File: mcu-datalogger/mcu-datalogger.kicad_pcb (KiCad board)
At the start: 2 copper layers, 29 parts, among them J1 Conn_01x04_Pin, J2 Conn_01x04_Pin, J3 Conn_01x09_Pin, J4 Conn_02x03_Odd_Even, U1 24LC1025, U2 24LC1025, U3 DS1337S_, U4 ATMEGA328P-AU, Y1 16MHz, Y2 32.768 KHz

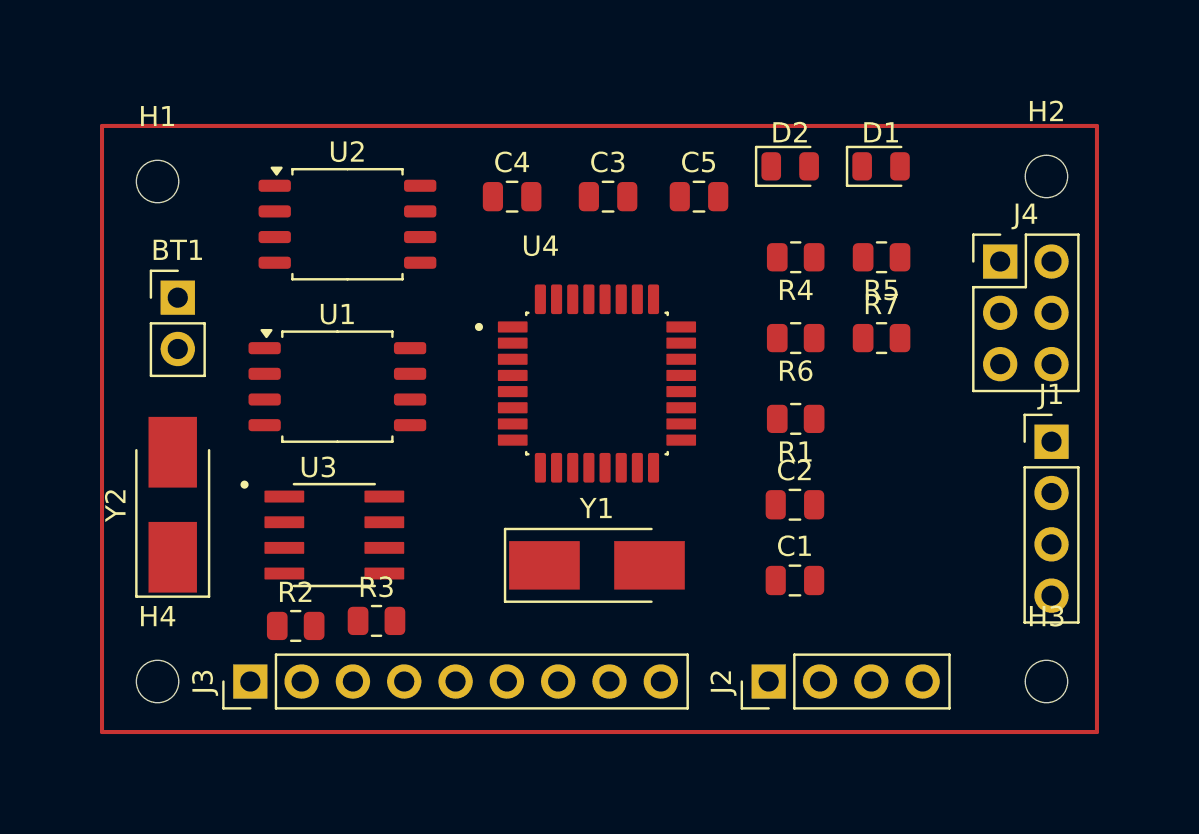
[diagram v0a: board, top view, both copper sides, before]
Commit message: routed pcb
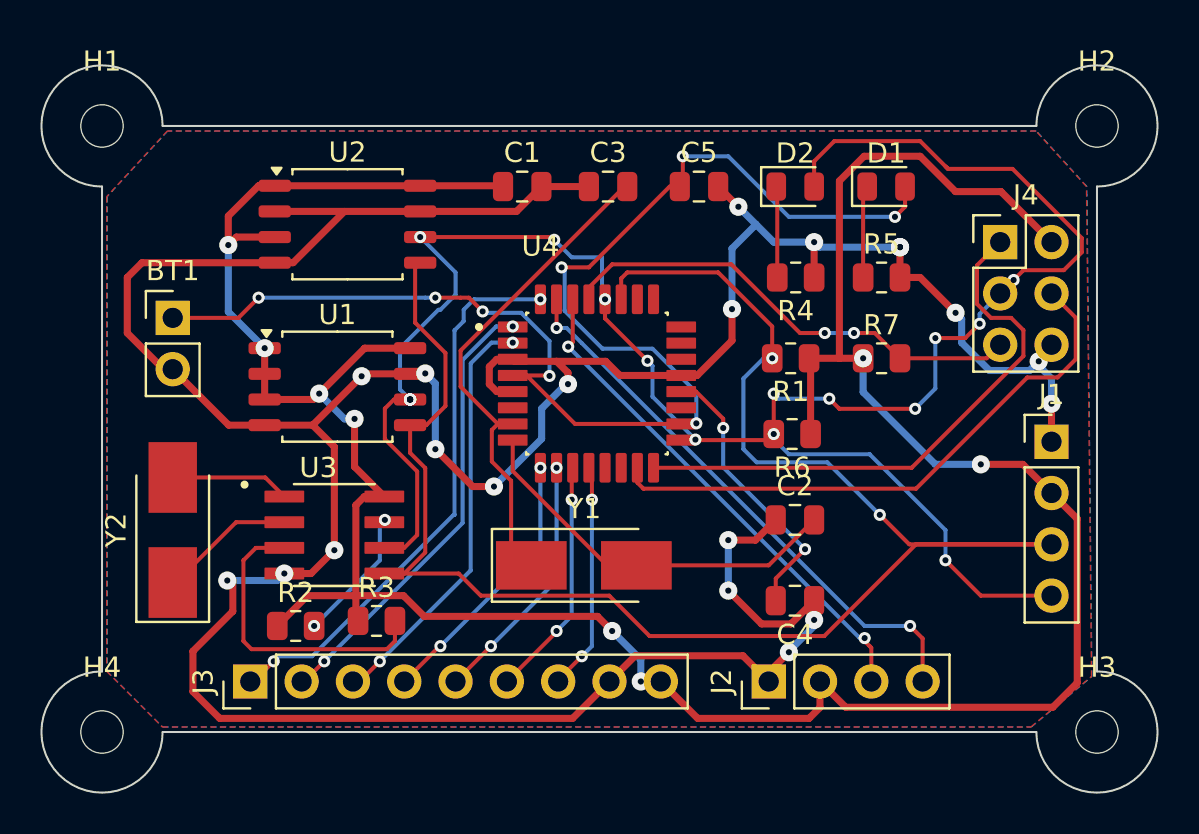
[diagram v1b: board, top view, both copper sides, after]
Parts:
- moved C4 24.4 mm to (92.0, 90.0), turned to 180 degrees
- moved C1 23.7 mm to (78.5, 69.5)
- moved R6 4.75 mm to (91.9, 81.8)
- moved H1 3.89 mm to (57.8, 66.5)
- moved H4 3.72 mm to (57.8, 96.5)
- moved H2 3.54 mm to (107.0, 66.5)
- moved H3 3.54 mm to (107.0, 96.5)
- moved R1 3.01 mm to (91.8, 78.0)
- moved Y2 1.25 mm to (61.2, 86.5)
- moved BT1 1.03 mm to (61.2, 76.0)
- moved D1 1.03 mm to (96.6, 69.5)
- moved D2 1.03 mm to (92.1, 69.5)
- moved R4 1.00 mm to (92.1, 74.0)
- moved R5 1.00 mm to (96.3, 74.0), turned to 0 degrees
- moved R7 1.00 mm to (96.3, 78.0)
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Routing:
- net GND: track 0.00 -> 180.9 mm, vias 0 -> 20
- net /Vcc: track 0.00 -> 145.8 mm, vias 0 -> 8
- net /SCK: track 0.00 -> 104.8 mm, vias 0 -> 17
- net /SDA: track 0.00 -> 89.1 mm, vias 0 -> 2
- net Net-(BT1-+): track 0.00 -> 67.5 mm, vias 0 -> 8
- net /MOSI: track 0.00 -> 29.0 mm
- net /TX: track 0.00 -> 28.6 mm, vias 0 -> 2
- net /MISO: track 0.00 -> 28.3 mm
- net /D2: track 0.00 -> 27.9 mm, vias 0 -> 2
- net /RX: track 0.00 -> 25.6 mm, vias 0 -> 2
- net Net-(U4-PB6): track 0.00 -> 24.7 mm
- net /RESET: track 0.00 -> 23.6 mm, vias 0 -> 2
- net /D3: track 0.00 -> 22.5 mm, vias 0 -> 2
- net /D4: track 0.00 -> 20.9 mm, vias 0 -> 2
- net Net-(U4-PB7): track 0.00 -> 19.3 mm
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- added copper zone on F.Cu, net /Vcc
- added copper zone on B.Cu, net GND
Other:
- board outline added: 55.2 x 36 mm
